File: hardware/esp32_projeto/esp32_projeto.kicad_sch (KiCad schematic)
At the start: 22 parts, among them J1 Conn_01x02, J2 Conn_01x04, U1 sdCard_adapter, U2 TP4056, U3 Oled_I2C_display, U4 ESP32-DEVKIT-V1, U5 ENS210, U6 DHT11

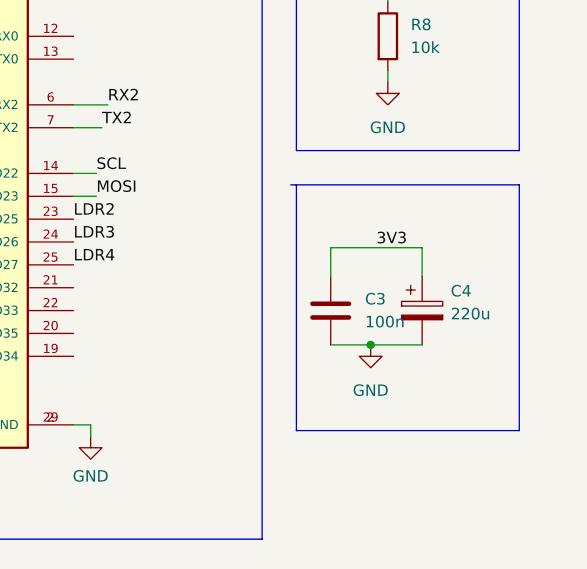
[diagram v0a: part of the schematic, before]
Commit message: change schematic
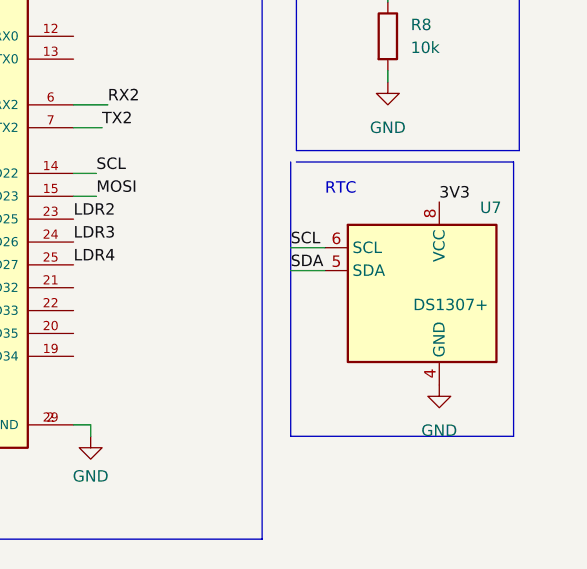
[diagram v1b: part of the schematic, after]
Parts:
- removed C3: 100n, symbol Device:C
- removed C4: 220u, symbol Device:C_Polarized
- added U7: DS1307+, Package_DIP:DIP-8_W7.62mm, symbol Timer_RTC:DS1307+
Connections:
- net 3V3: now also U7.8 (VCC)
- net GND: now also U7.4 (GND)
- net SCL: now also U7.6 (SCL)
- net SDA: now also U7.5 (SDA)
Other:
- note added: "RTC"
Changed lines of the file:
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@@
   (junction (at 107.315 39.37) (diameter 0) (color 0 0 0 0)
   )
-  (junction (at 150.495 146.05) (diameter 0) (color 0 0 0 0)
-  )
-  (polyline (pts (xy 142.24 128.27) (xy 167.005 128.27))
-    (stroke (width 0) (type default) (color 0 0 0 0))
-  )
   (polyline (pts (xy 136.525 80.01) (xy 136.525 50.165))
     (stroke (width 0) (type default) (color 0 0 0 0))
@@
     (stroke (width 0) (type default) (color 0 0 0 0))
   )
+  (wire (pts (xy 141.605 135.255) (xy 145.415 135.255))
+    (stroke (width 0) (type default) (color 0 0 0 0))
+  )
   (wire (pts (xy 57.785 111.76) (xy 60.325 111.76))
     (stroke (width 0) (type default) (color 0 0 0 0))
   )
-  (wire (pts (xy 156.21 138.43) (xy 156.21 135.255))
-    (stroke (width 0) (type default) (color 0 0 0 0))
-  )
-  (polyline (pts (xy 142.24 155.575) (xy 142.24 128.27))
-    (stroke (width 0) (type default) (color 0 0 0 0))
-  )
   (wire (pts (xy 24.765 27.94) (xy 27.94 27.94))
     (stroke (width 0) (type default) (color 0 0 0 0))
@@
     (stroke (width 0) (type default) (color 0 0 0 0))
   )
+  (polyline (pts (xy 166.37 156.21) (xy 141.605 156.21))
+    (stroke (width 0) (type default) (color 0 0 0 0))
+  )
   (polyline (pts (xy 72.39 81.28) (xy 72.39 167.64))
     (stroke (width 0) (type default) (color 0 0 0 0))
@@
     (stroke (width 0) (type default) (color 0 0 0 0))
   )
-  (wire (pts (xy 146.05 135.255) (xy 156.21 135.255))
-    (stroke (width 0) (type default) (color 0 0 0 0))
-  )
   (polyline (pts (xy 41.275 131.445) (xy 66.04 131.445))
     (stroke (width 0) (type default) (color 0 0 0 0))
@@
     (stroke (width 0) (type default) (color 0 0 0 0))
   )
-  (polyline (pts (xy 141.605 128.27) (xy 142.24 128.27))
-    (stroke (width 0) (type default) (color 0 0 0 0))
-  )
   (wire (pts (xy 51.435 139.065) (xy 51.435 140.335))
     (stroke (width 0) (type default) (color 0 0 0 0))
@@
     (stroke (width 0) (type default) (color 0 0 0 0))
   )
-  (polyline (pts (xy 167.005 128.27) (xy 167.005 155.575))
-    (stroke (width 0) (type default) (color 0 0 0 0))
-  )
   (wire (pts (xy 82.55 147.32) (xy 86.995 147.32))
     (stroke (width 0) (type default) (color 0 0 0 0))
@@
     (stroke (width 0) (type default) (color 0 0 0 0))
   )
+  (polyline (pts (xy 141.605 125.73) (xy 141.605 156.21))
+    (stroke (width 0) (type default) (color 0 0 0 0))
+  )
   (wire (pts (xy 51.435 147.955) (xy 51.435 152.4))
     (stroke (width 0) (type default) (color 0 0 0 0))
@@
     (stroke (width 0) (type default) (color 0 0 0 0))
   )
-  (wire (pts (xy 146.05 138.43) (xy 146.05 135.255))
+  (polyline (pts (xy 166.37 125.73) (xy 166.37 156.21))
     (stroke (width 0) (type default) (color 0 0 0 0))
   )
@@
     (stroke (width 0) (type default) (color 0 0 0 0))
   )
-  (wire (pts (xy 146.05 146.05) (xy 150.495 146.05))
-    (stroke (width 0) (type default) (color 0 0 0 0))
-  )
   (wire (pts (xy 24.13 160.02) (xy 24.13 161.29))
     (stroke (width 0) (type default) (color 0 0 0 0))
@@
     (stroke (width 0) (type default) (color 0 0 0 0))
   )
-  (polyline (pts (xy 167.005 155.575) (xy 142.24 155.575))
-    (stroke (width 0) (type default) (color 0 0 0 0))
-  )
   (wire (pts (xy 57.785 106.68) (xy 60.325 106.68))
     (stroke (width 0) (type default) (color 0 0 0 0))
@@
     (stroke (width 0) (type default) (color 0 0 0 0))
   )
-  (wire (pts (xy 156.21 146.05) (xy 150.495 146.05))
+  (polyline (pts (xy 142.24 125.73) (xy 166.37 125.73))
     (stroke (width 0) (type default) (color 0 0 0 0))
   )
@@
   )
   (wire (pts (xy 78.74 36.195) (xy 78.74 40.005))
+    (stroke (width 0) (type default) (color 0 0 0 0))
+  )
+  (wire (pts (xy 141.605 137.795) (xy 145.415 137.795))
     (stroke (width 0) (type default) (color 0 0 0 0))
   )
@@
     (effects (font (size 3 3)) (justify left bottom))
   )
+  (text "RTC\n" (at 145.415 129.54 0)
+    (effects (font (size 1.27 1.27)) (justify left bottom))
+  )
   (label "3V3" (at 24.13 139.065 0)
     (effects (font (size 1.27 1.27)) (justify left bottom))
@@
     (effects (font (size 1.27 1.27)) (justify left bottom))
   )
+  (label "SDA" (at 141.605 137.795 0)
+    (effects (font (size 1.27 1.27)) (justify left bottom))
+  )
   (label "3V3" (at 45.72 57.785 0)
     (effects (font (size 1.27 1.27)) (justify left bottom))
@@
     (effects (font (size 1.27 1.27)) (justify left bottom))
   )
+  (label "3V3" (at 158.115 130.175 0)
+    (effects (font (size 1.27 1.27)) (justify left bottom))
+  )
   (label "MOSI" (at 120.015 129.54 0)
     (effects (font (size 1.27 1.27)) (justify left bottom))
@@
     (effects (font (size 1.27 1.27)) (justify left bottom))
   )
+  (label "SCL" (at 141.605 135.255 0)
+    (effects (font (size 1.27 1.27)) (justify left bottom))
+  )
   (label "LDR1" (at 81.28 139.065 0)
     (effects (font (size 1.27 1.27)) (justify left bottom))
   )
   (label "CS" (at 60.325 101.6 0)
-    (effects (font (size 1.27 1.27)) (justify left bottom))
-  )
-  (label "3V3" (at 151.13 135.255 0)
     (effects (font (size 1.27 1.27)) (justify left bottom))
   )
@@
     (pin "2")
   )
+  (symbol (lib_id "power:GND") (at 158.115 150.495 0) (unit 1)
+    (in_bom yes) (on_board yes) (fields_autoplaced)
+    (property "Reference" "#PWR011" (id 0) (at 158.115 156.845 0)
+      (effects (font (size 1.27 1.27)) hide)
+    )
+    (property "Value" "GND" (id 1) (at 158.115 155.575 0))
+    (property "Footprint" "" (id 2) (at 158.115 150.495 0)
+      (effects (font (size 1.27 1.27)) hide)
+    )
+    (property "Datasheet" "" (id 3) (at 158.115 150.495 0)
+      (effects (font (size 1.27 1.27)) hide)
+    )
+    (pin "1")
+  )
   (symbol (lib_id "power:GND") (at 119.38 156.21 0) (unit 1)
     (in_bom yes) (on_board yes) (fields_autoplaced)
@@
     )
     (pin "1")
-  )
-  (symbol (lib_id "Device:C") (at 146.05 142.24 0) (unit 1)
-    (in_bom yes) (on_board yes) (fields_autoplaced)
-    (property "Reference" "C3" (id 0) (at 149.86 140.9699 0)
-      (effects (font (size 1.27 1.27)) (justify left))
-    )
-    (property "Value" "100n" (id 1) (at 149.86 143.5099 0)
-      (effects (font (size 1.27 1.27)) (justify left))
-    )
-    (property "Footprint" "" (id 2) (at 147.0152 146.05 0)
-      (effects (font (size 1.27 1.27)) hide)
-    )
-    (property "Datasheet" "~" (id 3) (at 146.05 142.24 0)
-      (effects (font (size 1.27 1.27)) hide)
-    )
-    (pin "1")
-    (pin "2")
   )
   (symbol (lib_id "Sensor_Humidity:ENS210") (at 116.205 64.135 0) (unit 1)
@@
     (pin "1")
   )
+  (symbol (lib_id "Timer_RTC:DS1307+") (at 158.115 140.335 0) (unit 1)
+    (in_bom yes) (on_board yes)
+    (property "Reference" "U7" (id 0) (at 163.83 130.81 0))
+    (property "Value" "DS1307+" (id 1) (at 159.385 141.605 0))
+    (property "Footprint" "Package_DIP:DIP-8_W7.62mm" (id 2) (at 158.115 153.035 0)
+      (effects (font (size 1.27 1.27)) hide)
+    )
+    (property "Datasheet" "https://datasheets.maximintegrated.com/en/ds/DS1307.pdf" (id 3) (at 158.115 145.415 0)
+      (effects (font (size 1.27 1.27)) hide)
+    )
+    (pin "4")
+    (pin "5")
+    (pin "6")
+    (pin "8")
+  )
   (symbol (lib_id "power:GND") (at 118.745 71.755 0) (unit 1)
     (in_bom yes) (on_board yes) (fields_autoplaced)
@@
     )
     (property "Datasheet" "" (id 3) (at 118.745 71.755 0)
-      (effects (font (size 1.27 1.27)) hide)
-    )
-    (pin "1")
-  )
-  (symbol (lib_id "power:GND") (at 150.495 146.05 0) (unit 1)
-    (in_bom yes) (on_board yes) (fields_autoplaced)
-    (property "Reference" "#PWR011" (id 0) (at 150.495 152.4 0)
-      (effects (font (size 1.27 1.27)) hide)
-    )
-    (property "Value" "GND" (id 1) (at 150.495 151.13 0))
-    (property "Footprint" "" (id 2) (at 150.495 146.05 0)
-      (effects (font (size 1.27 1.27)) hide)
-    )
-    (property "Datasheet" "" (id 3) (at 150.495 146.05 0)
       (effects (font (size 1.27 1.27)) hide)
     )
@@
     (pin "1")
   )
-  (symbol (lib_id "Device:C_Polarized") (at 156.21 142.24 0) (unit 1)
-    (in_bom yes) (on_board yes) (fields_autoplaced)
-    (property "Reference" "C4" (id 0) (at 159.385 140.0809 0)
-      (effects (font (size 1.27 1.27)) (justify left))
-    )
-    (property "Value" "220u" (id 1) (at 159.385 142.6209 0)
-      (effects (font (size 1.27 1.27)) (justify left))
-    )
-    (property "Footprint" "" (id 2) (at 157.1752 146.05 0)
-      (effects (font (size 1.27 1.27)) hide)
-    )
-    (property "Datasheet" "~" (id 3) (at 156.21 142.24 0)
-      (effects (font (size 1.27 1.27)) hide)
-    )
-    (pin "1")
-    (pin "2")
-  )
   (symbol (lib_id "power:GND") (at 60.325 115.57 0) (unit 1)
     (in_bom yes) (on_board yes) (fields_autoplaced)
@@
       (reference "#PWR010") (unit 1) (value "GND") (footprint "")
     )
-    (path "/97b512c1-f596-492a-93b8-ce5fd4a98f72"
+    (path "/3ed32a49-2f42-47c6-a219-2bc323543d3b"
       (reference "#PWR011") (unit 1) (value "GND") (footprint "")
     )
@@
       (reference "C2") (unit 1) (value "470u") (footprint "")
     )
-    (path "/4bc41f4c-1c6f-43de-8d90-f4ce906c22ea"
-      (reference "C3") (unit 1) (value "100n") (footprint "")
-    )
-    (path "/c41574a1-04bd-494b-aeb1-1a66e0e0380a"
-      (reference "C4") (unit 1) (value "220u") (footprint "")
-    )
     (path "/a2358ef7-a54e-4cdf-8c1c-4491dbf175ac"
       (reference "J1") (unit 1) (value "Conn_01x02") (footprint "")
@@
       (reference "U6") (unit 1) (value "DHT11") (footprint "Sensor:Aosong_DHT11_5.5x12.0_P2.54mm")
     )
-  )
+    (path "/8d2b2424-5bb3-42bc-bd25-295e03e5bdce"
+      (reference "U7") (unit 1) (value "DS1307+") (footprint "Package_DIP:DIP-8_W7.62mm")
+    )
+  )
